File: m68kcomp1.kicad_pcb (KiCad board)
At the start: 2 copper layers, 159.5 x 99.8 mm, 55 parts, among them P1 CONN_CTL_DATA, P2 CONN_ADDR, P3 POWER, SW1 RST_SW, SW2 PWR_SW, U1 74LS04, U10 sram_um61512ak, U11 sram_um61512ak, U12 68010D, U13 at28c64, U14 NE555, U15 sram_um61512ak, U16 sram_um61512ak, U2 74LS08, U3 74LS32, U4 74HC05, U5 address_decoder, U6 74HC04, U7 74HC74, U8 74LS148, U9 at28c64, Y1 20MHz

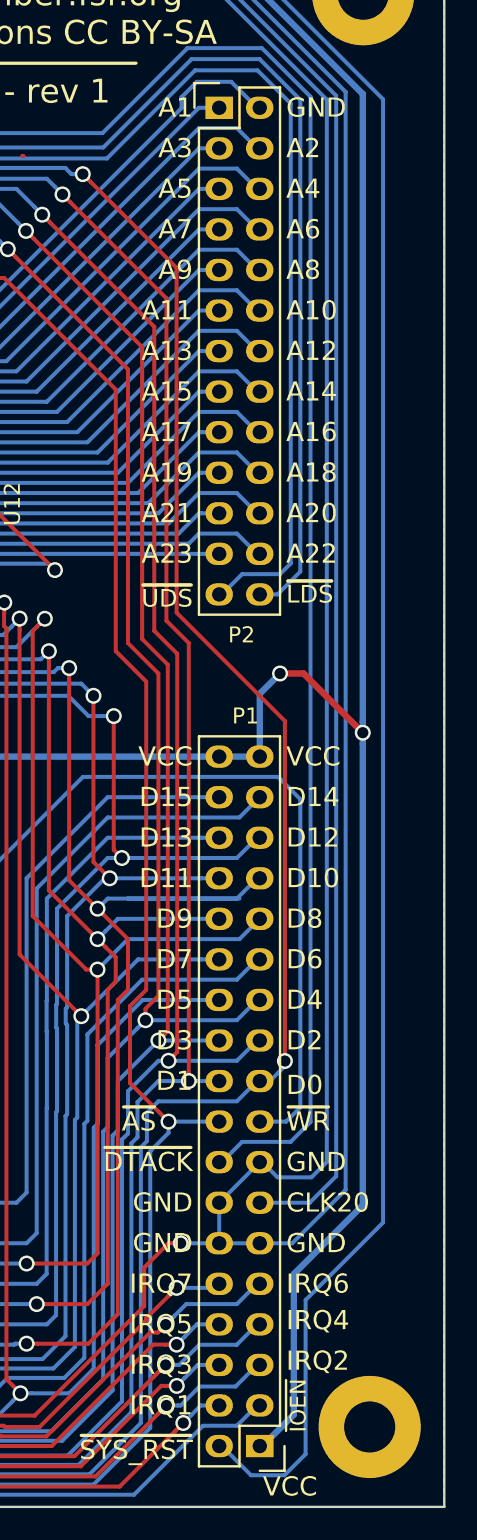
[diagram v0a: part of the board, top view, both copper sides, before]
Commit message: changes for manufacture
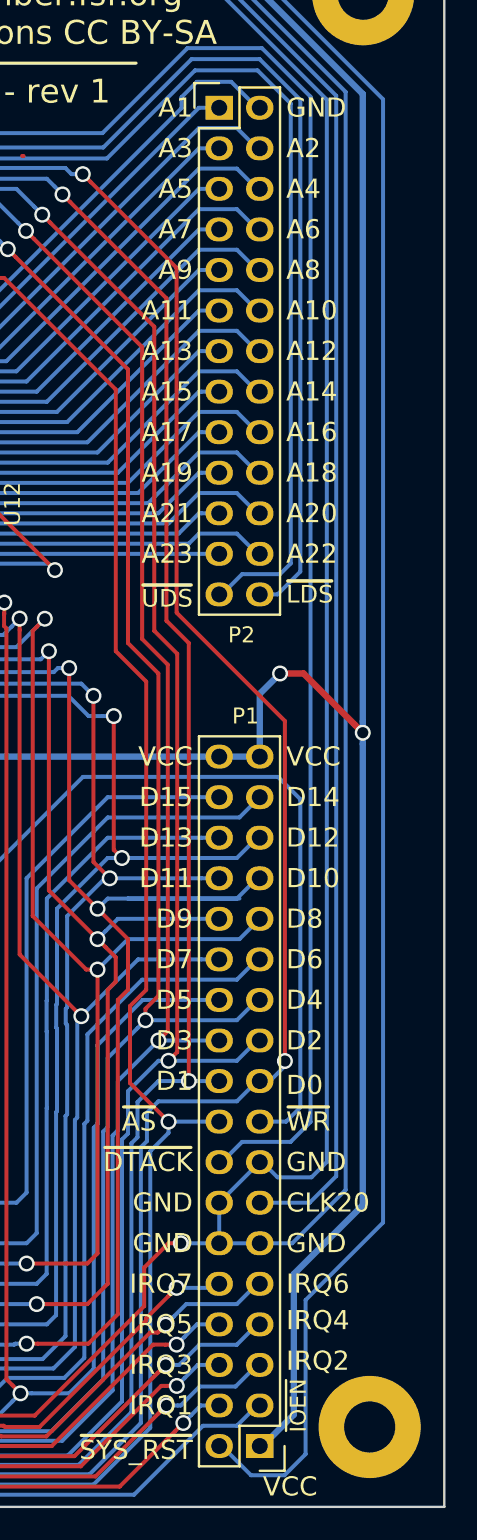
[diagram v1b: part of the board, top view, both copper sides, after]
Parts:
- P1: footprint m68kcomp1:Pin_Header_Straight_2x18 -> Pin_Header_Straight_2x18
- P2: footprint m68kcomp1:Pin_Header_Straight_2x13_oval -> Pin_Header_Straight_2x13_oval
